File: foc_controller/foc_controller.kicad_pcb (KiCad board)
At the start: 2 copper layers, 34 x 26.5 mm, 46 parts, among them J1 Conn_01x02, J1-Programmer1 Conn_01x05, J2 Conn_01x04, J3 Conn_01x03, J5 USB_C_Receptacle_USB2.0_16P, J6 Conn_01x02, U1 AZ1117-3.3, U2 INA4180A2IPWR, U4 AS5048B, U5 STM32G431KBUx, Y1 16MHz

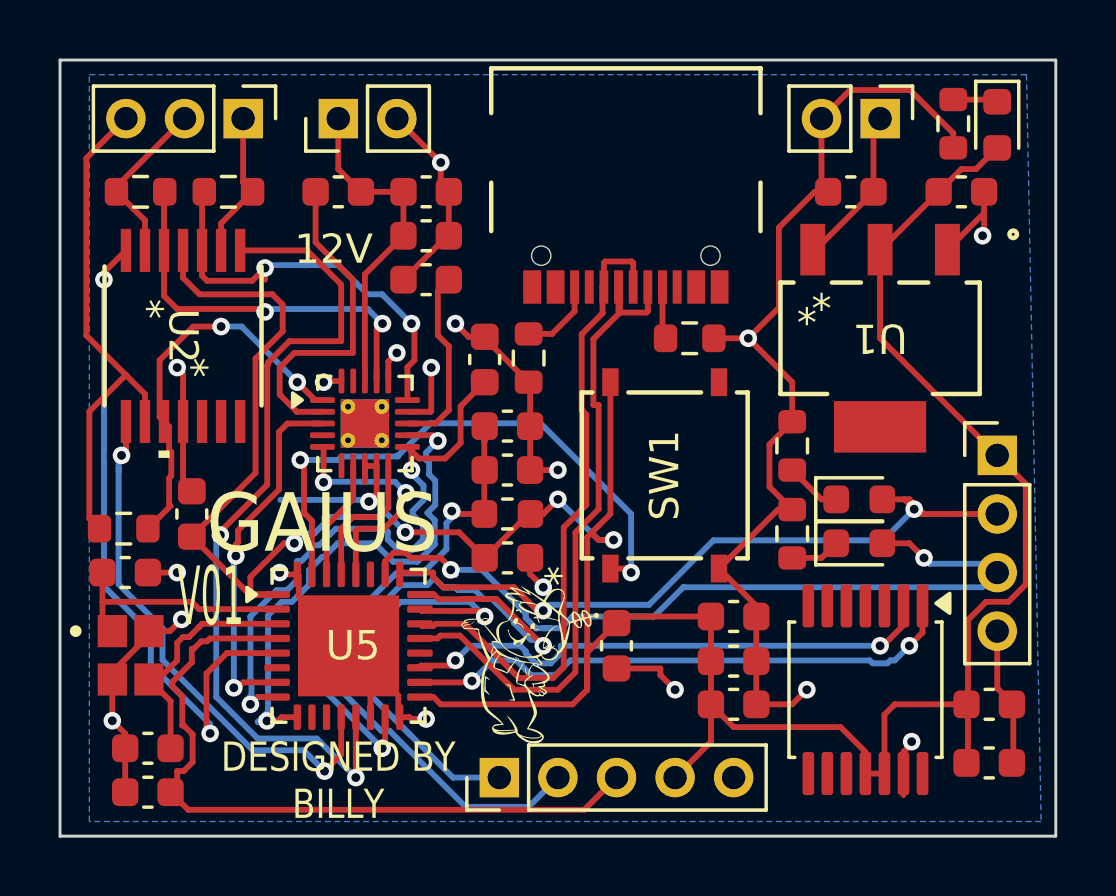
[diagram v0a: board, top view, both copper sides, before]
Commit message: Commiting again
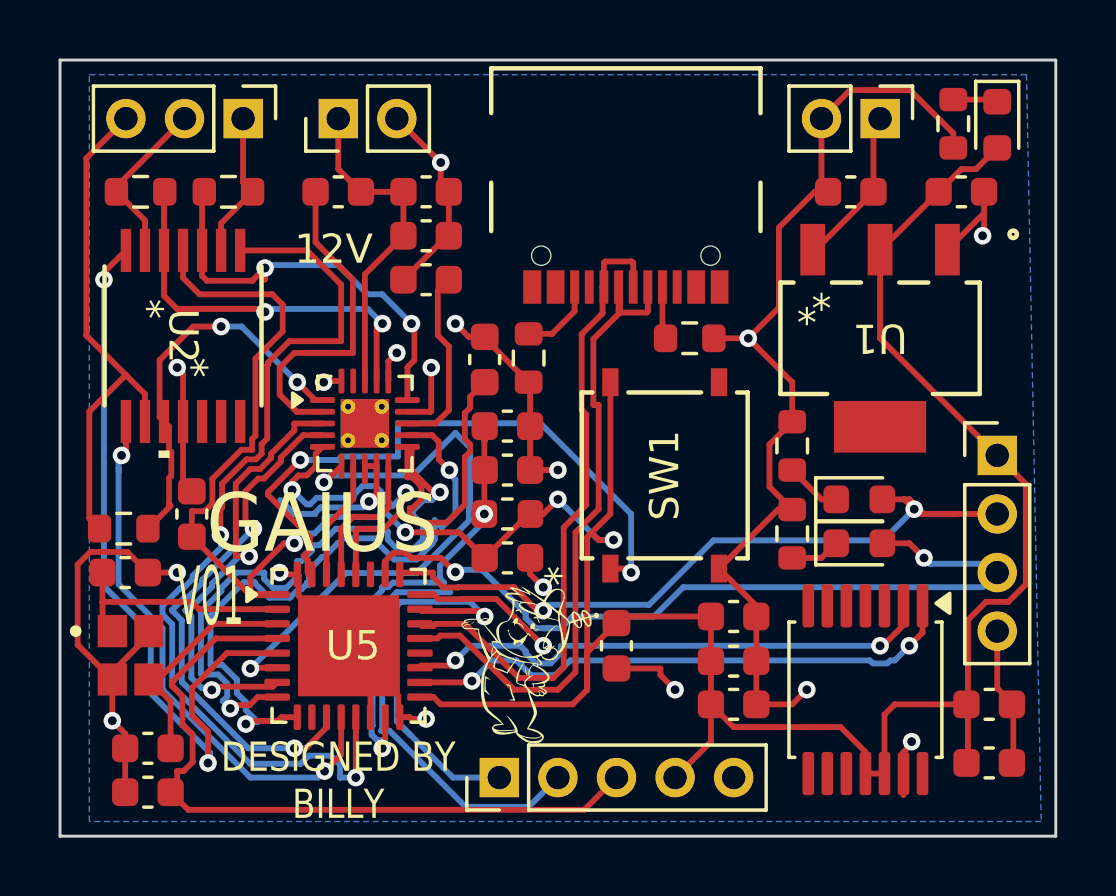
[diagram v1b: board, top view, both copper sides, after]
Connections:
- U3 pad 6: PA2_TIM15_CH1N -> PA1_TIM15_CH1N
- U5 pad 11: PA6_TIM15_CH1 -> PA6_TIM16_CH1
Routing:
- net PA1_TIM15_CH1N: track 0.00 -> 19.7 mm, vias 0 -> 2
- net PA6_TIM16_CH1: track 0.00 -> 18.0 mm, vias 0 -> 2
- net MOTOR_STDBY: track 20.6 -> 30.9 mm
- net GND: track 95.0 -> 101.4 mm, vias 19 -> 18
- net Net-(J1-Programmer1-Pin_2): track 24.9 -> 19.6 mm
- net MOTOR_DIAG: track 17.9 -> 22.7 mm
- net PA2_TIM15_CH1: track 12.6 -> 15.7 mm
- net U_ADC1_IN15: track 29.2 -> 32.2 mm
- net PB5_TIM17_CH1: track 8.26 -> 11.1 mm
- net V_ADC1_IN10: track 23.1 -> 25.5 mm
- net Net-(SW1-B): track 20.0 -> 21.8 mm
- net Net-(J1-Programmer1-Pin_1): track 15.4 -> 14.2 mm
- net +3.3VA: track 16.5 -> 15.4 mm
- net W_ADC2_IN4: track 18.1 -> 18.8 mm
